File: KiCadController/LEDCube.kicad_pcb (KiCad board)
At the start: 4 copper layers, 56 parts, among them IC100 MCP73833T-FCI_MF, IC101 CP2102N-A02-GQFN28, IC102 ESP32-WROOM-32E-H4, J100 1769, J102 USB4110-GF-A, J103 15-91-0100, J104 15-91-0100, J105 15-91-0100, J106 15-91-0100, J107 15-91-0100, J108 15-91-0100, Q100 Q_NMOS_GSD, Q101 Q_NMOS_GSD, Q102 Q_NMOS_GSD, Q103 Q_NMOS_GSD, Q104 Q_NMOS_GSD

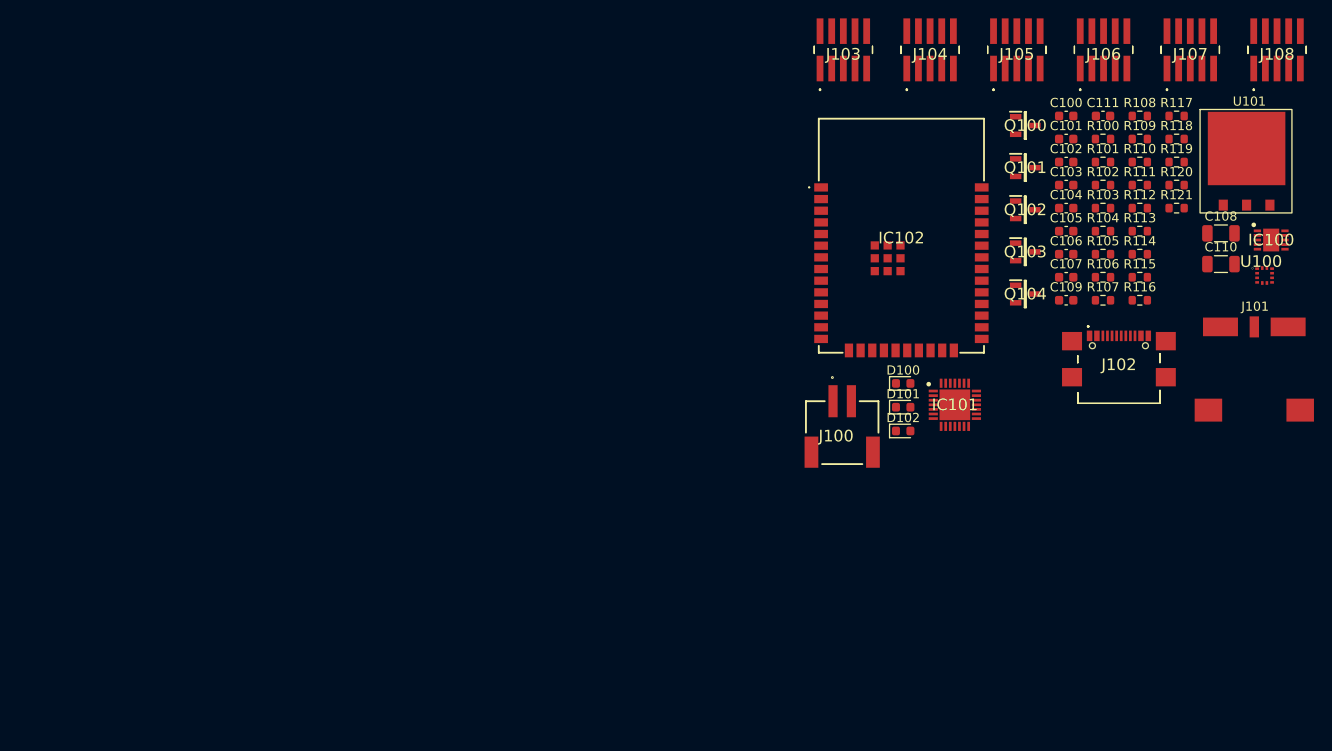
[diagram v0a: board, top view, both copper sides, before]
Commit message: Update for MTE
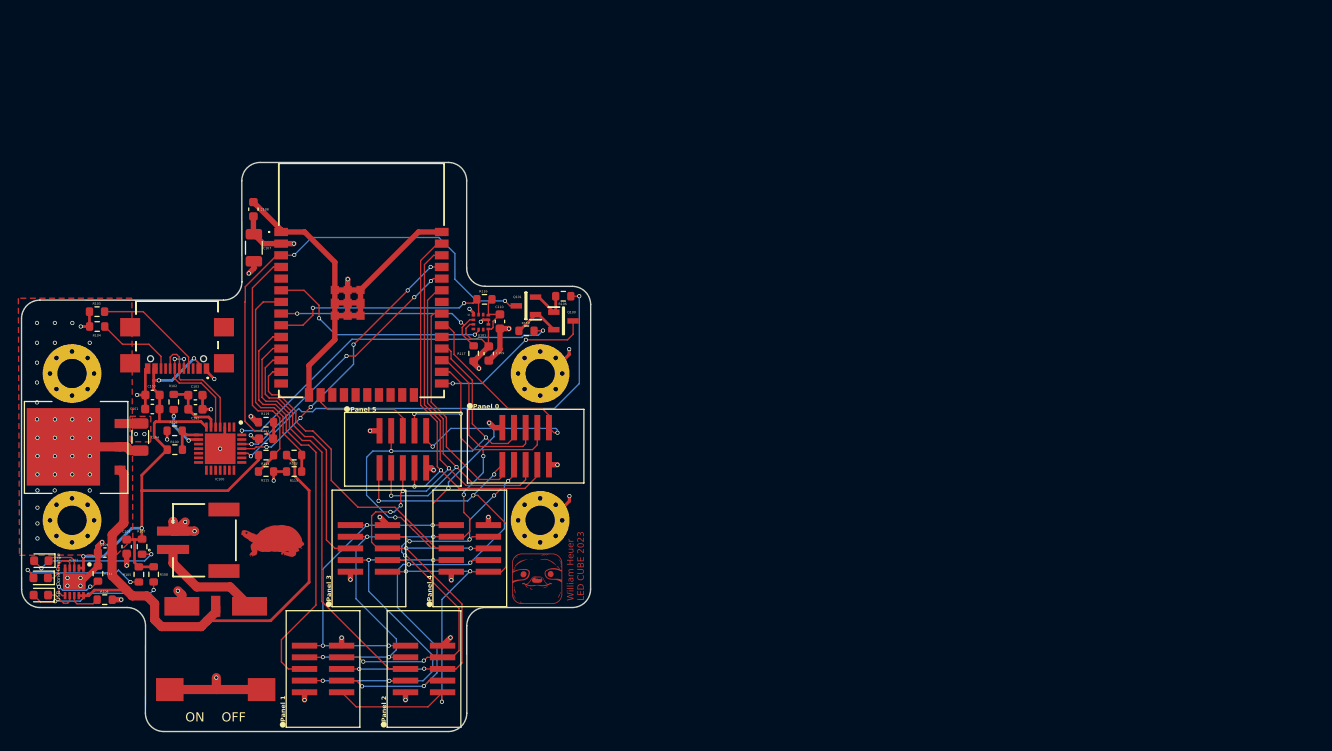
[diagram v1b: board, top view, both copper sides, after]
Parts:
- removed the Q100 at (208.8, 47.7)
- removed the Q101 at (208.8, 52.3)
- removed Q102: Q_NMOS_GSD, SamacSys_Parts:SOT96P237X111-3N
- removed the R104 at (217.3, 59.2)
- removed the R105 at (217.3, 61.8)
- removed the R106 at (217.3, 64.3)
- removed the R117 at (225.3, 46.7)
- added G***: LOGO, LOGO, F.Cu at (155.6, 97.1)
- added G***: LOGO, LOGO, F.Cu at (126.8, 93.0)
- added H100: MountingHole, MountingHole:MountingHole_3.2mm_M3_Pad_Via, F.Cu at (105.0, 74.8)
- added H101: MountingHole, MountingHole:MountingHole_3.2mm_M3_Pad_Via, F.Cu at (155.9, 74.8)
- added H102: MountingHole, MountingHole:MountingHole_3.2mm_M3_Pad_Via, F.Cu at (105.0, 90.8)
- added H103: MountingHole, MountingHole:MountingHole_3.2mm_M3_Pad_Via, F.Cu at (155.9, 90.8)
- added R111: 2k, Resistor_SMD:R_0603_1608Metric, F.Cu at (107.8, 96.5)
- J103: renamed from J106; footprint SamacSys_Parts:FTSH10501FDVK -> LEDCube:CNC_TECH_SMD_10POS
- J104: renamed from J103; footprint SamacSys_Parts:FTSH10501FDVK -> LEDCube:CNC_TECH_SMD_10POS
- J105: renamed from J108; footprint SamacSys_Parts:FTSH10501FDVK -> LEDCube:CNC_TECH_SMD_10POS
- J106: renamed from J105; footprint SamacSys_Parts:FTSH10501FDVK -> LEDCube:CNC_TECH_SMD_10POS
- J107: footprint SamacSys_Parts:FTSH10501FDVK -> LEDCube:CNC_TECH_SMD_10POS
- J108: renamed from J104; footprint SamacSys_Parts:FTSH10501FDVK -> LEDCube:CNC_TECH_SMD_10POS
- moved IC101 135.6 mm to (105.2, 97.5), turned to -90 degrees
- moved U100 125.5 mm to (110.2, 82.7), turned to 90 degrees
- moved C104 119.2 mm to (112.4, 81.7), turned to -90 degrees
- moved R103 118.4 mm to (107.7, 68.0), turned to 180 degrees
- moved R104 118.3 mm to (107.7, 69.6), turned to 180 degrees
- moved J101 117.2 mm to (120.6, 100.1)
- moved R105 115.3 mm to (112.2, 96.6), turned to -90 degrees
- moved J105 114.6 mm to (135.3, 93.8), turned to 90 degrees
- moved R109 113.6 mm to (108.5, 99.4)
- moved R107 112.8 mm to (112.6, 93.6), turned to -90 degrees
- moved R108 111.8 mm to (113.8, 96.6), turned to -90 degrees
- moved R100 111.2 mm to (116.2, 83.0)
- moved C105 110.6 mm to (110.9, 93.6), turned to -90 degrees
- moved J103 110.1 mm to (130.3, 106.9), turned to 90 degrees
- moved R101 109.9 mm to (116.1, 81.0), turned to 180 degrees
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- renumbered C105 to C102, C106 to C103, C110 to C104, C102 to C105, C107 to C106, C108 to C107, C109 to C108, C103 to C109, C104 to C110, IC101 to IC100, IC100 to IC101, J102 to J100, J100 to J102, Q103 to Q100, Q104 to Q101, R108 to R100, R109 to R101, R103 to R102, R120 to R103, R121 to R104, R100 to R105, R112 to R106, R101 to R107, R102 to R108, R107 to R109, R113 to R110, R115 to R112, R118 to R113, R116 to R114, R119 to R115, R110 to R116, R111 to R117, R114 to R119, U101 to U100, U100 to U101
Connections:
- C111 pad 1: Net-(IC102-EN) -> EN
- IC100 pad 13: CHG_100mA -> unconnected-(IC100-CHREN-Pad13)
- IC100 pad 14: CHG_1.5A -> unconnected-(IC100-CHR1-Pad14)
- IC100 pad 15: CHG_500mA -> unconnected-(IC100-CHR0-Pad15)
- IC102 pad 27: MUX_B3 -> SERIAL_IN0
- IC102 pad 28: BRIGHTNESS_PWM -> MUX_B3
- IC102 pad 3: Net-(IC102-EN) -> EN
- IC102 pad 30: MUX_B0 -> LATCH
- IC102 pad 33: LATCH -> MASTER_CLK
- IC102 pad 36: MASTER_CLK -> MUX_B0
- IC102 pad 37: SERIAL_IN0 -> BRIGHTNESS_PWM
- IC102 pad 5: CHG_100mA -> unconnected-(IC102-SENSOR_VN-Pad5)
- R119 pad 2: Net-(IC102-EN) -> EN
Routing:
- net GND: track 0.00 -> 135.4 mm, vias 0 -> 64
- net MUX_B1: track 0.00 -> 95.7 mm, vias 0 -> 6
- net MUX_B0: track 0.00 -> 94.8 mm, vias 0 -> 8
- net BRIGHTNESS_PWM: track 0.00 -> 92.6 mm, vias 0 -> 8
- net MASTER_CLK: track 0.00 -> 91.5 mm, vias 0 -> 7
- net MUX_B3: track 0.00 -> 90.0 mm, vias 0 -> 7
- net LATCH: track 0.00 -> 86.9 mm, vias 0 -> 7
- net MUX_B2: track 0.00 -> 76.6 mm, vias 0 -> 8
- net VBUS: track 0.00 -> 64.1 mm, vias 0 -> 4
- net VBAT: track 0.00 -> 61.3 mm
- net EN: track 0.00 -> 56.8 mm, vias 0 -> 2
- net RTS: track 0.00 -> 50.9 mm, vias 0 -> 2
- net SERIAL_IN1: track 0.00 -> 45.2 mm
- net SERIAL_IN2: track 0.00 -> 45.0 mm
- net DTR: track 0.00 -> 38.8 mm, vias 0 -> 2
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- added copper zone on F.Cu, net +3V3
- added copper zone on In2.Cu, net +3V3
- added copper zone on F.Cu, net GND
- added copper zone on In1.Cu, net GND
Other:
- board outline added: 62 x 62 mm
- board text added: "C100"
- board text added: "C101"
- board text added: "C102"
- board text added: "C103"
- board text added: "C104"
- board text added: "C105"
- board text added: "C106"
- board text added: "C107"
- board text added: "C108"
- board text added: "C109"
- board text added: "C110"
- board text added: "C111"
- board text added: "Charge"
- board text added: "Done"
- board text added: "IC100"
- board text added: "IC101"
- board text added: "OFF"
- board text added: "ON"
- board text added: "Panel 0"
- board text added: "Panel 1"
- board text added: "Panel 2"
- board text added: "Panel 3"
- board text added: "Panel 4"
- board text added: "Panel 5"
- board text added: "Q100"
- board text added: "Q101"
- board text added: "R100"
- board text added: "R101"
- board text added: "R102"
- board text added: "R103"
- board text added: "R104"
- board text added: "R105"
- board text added: "R106"
- board text added: "R107"
- board text added: "R108"
- board text added: "R109"
- board text added: "R110"
- board text added: "R111"
- board text added: "R112"
- board text added: "R113"
- board text added: "R114"
- board text added: "R115"
- board text added: "R116"
- board text added: "R117"
- board text added: "R119"
- board text added: "U101"
- board text added: "USB"
- board text added: "William Heuer LED CUBE 2023"
